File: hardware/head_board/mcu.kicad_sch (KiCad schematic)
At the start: 49 parts, among them SW1 BOOTSEL, U3 RP2040, U4 TVS, U5 W25Q128JVS, U9 74HC2G34, Y1 12MHz

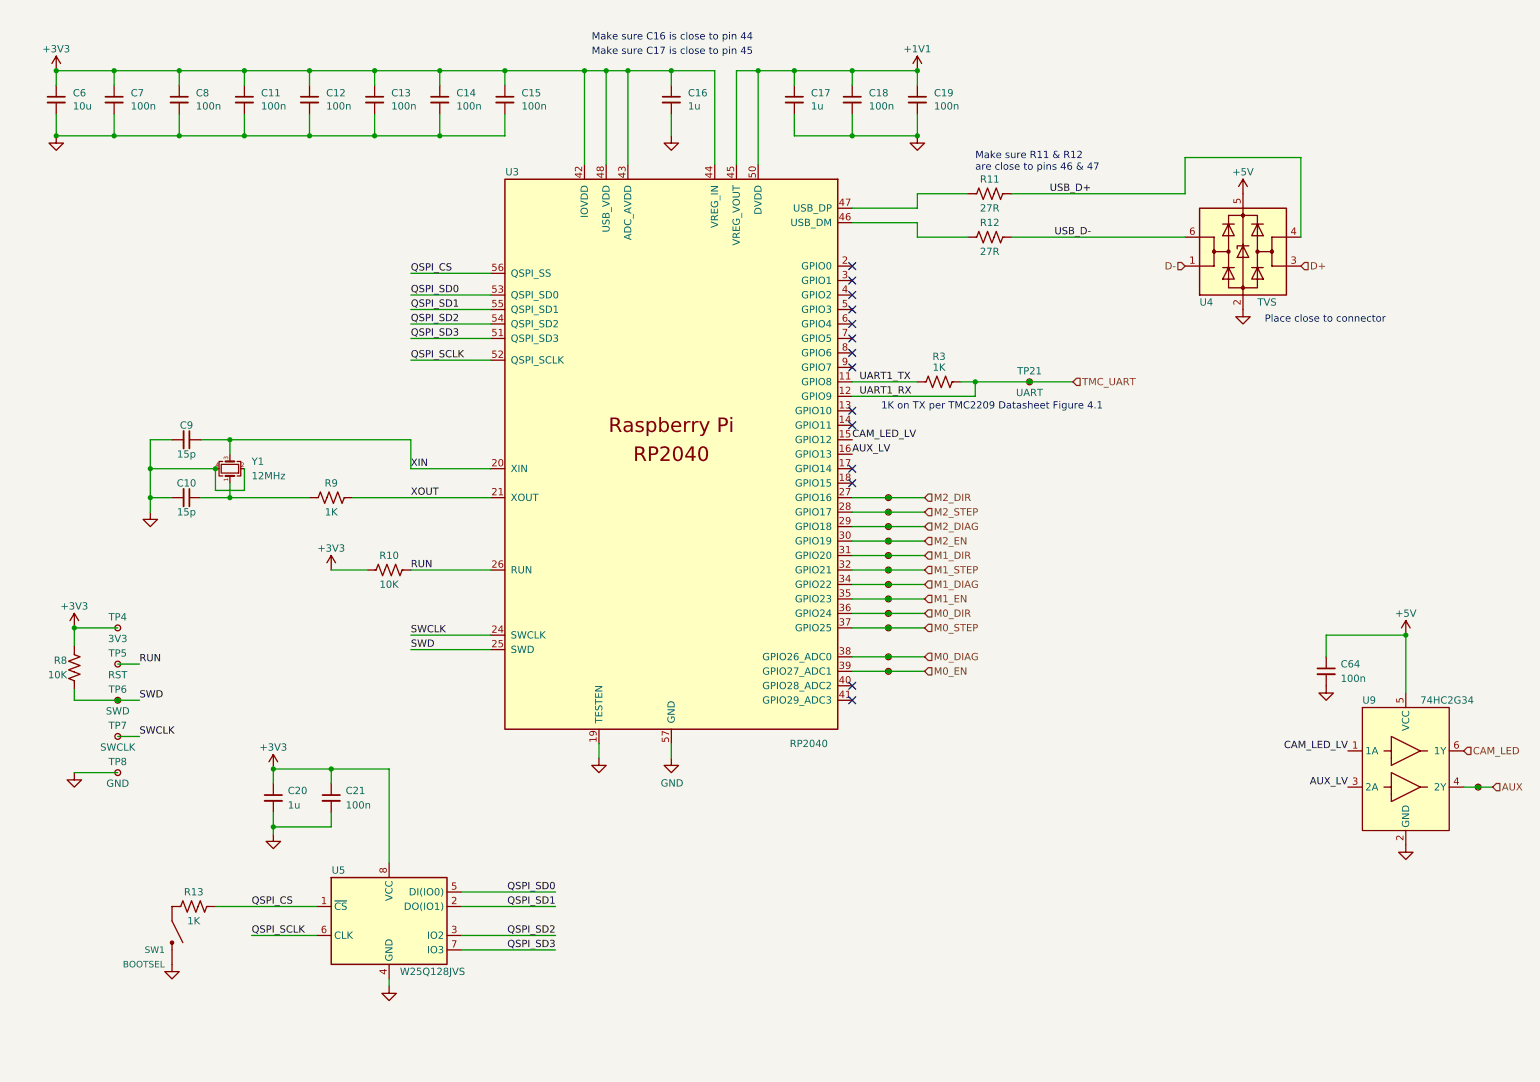
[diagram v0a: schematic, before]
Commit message: v1 revision to the schematic
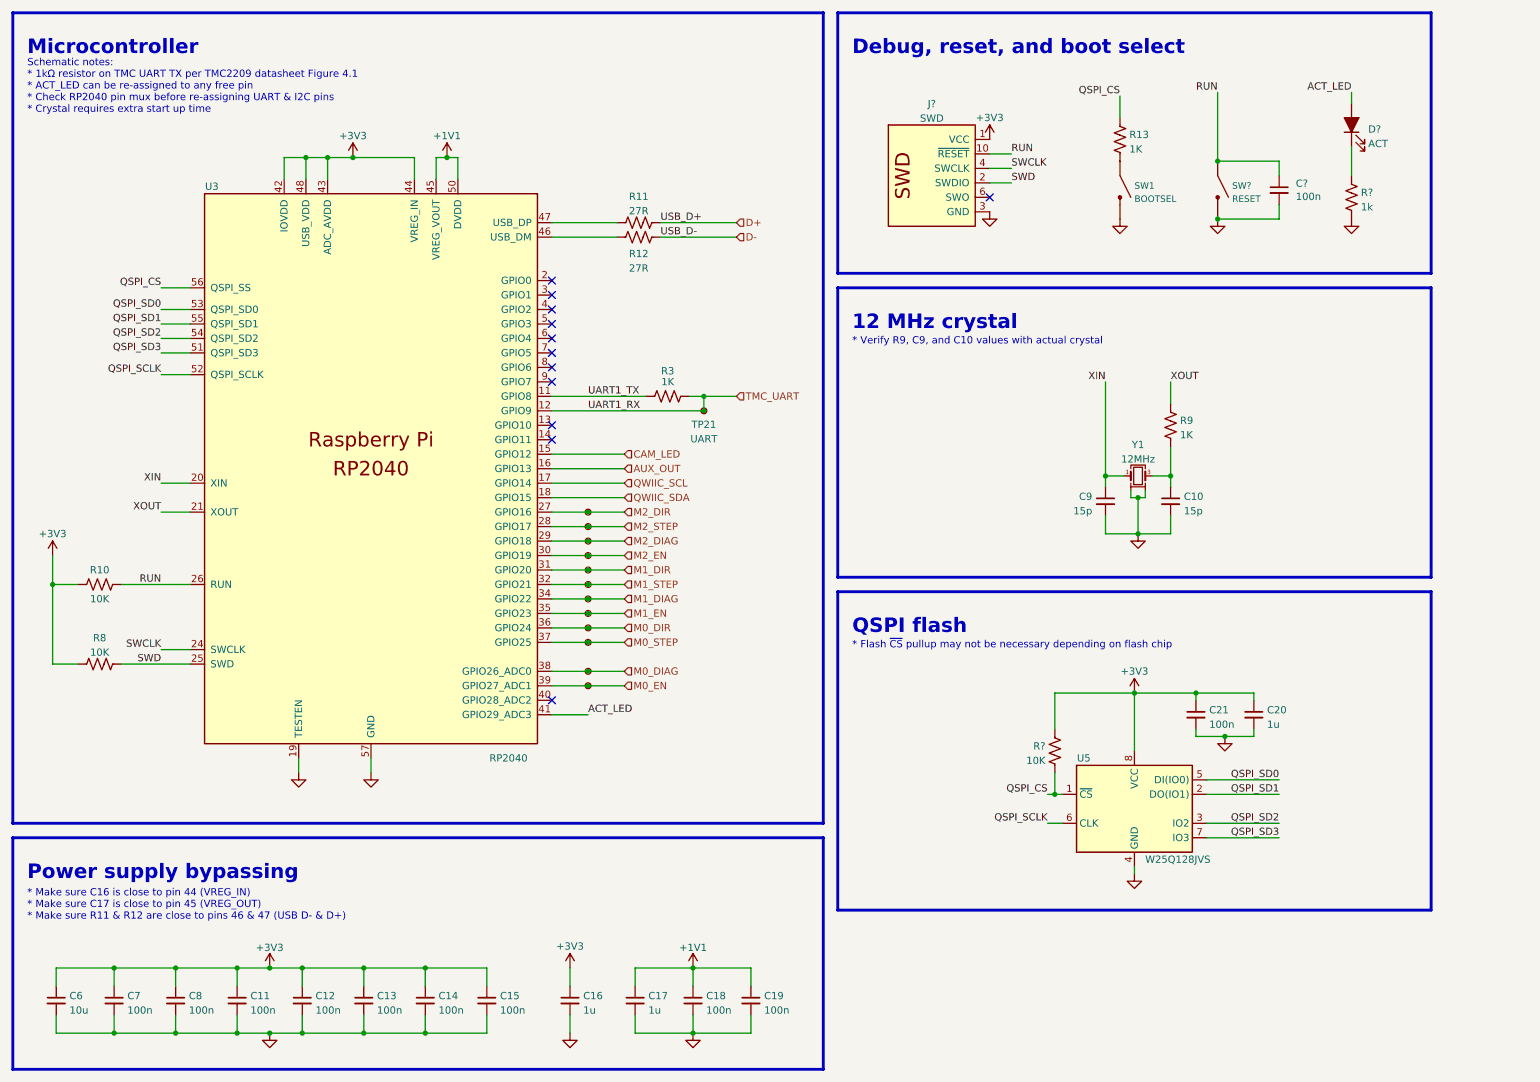
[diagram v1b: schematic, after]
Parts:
- removed C64: 100n, Capacitor_SMD:C_0402_1005Metric_Pad0.74x0.62mm_HandSolder, symbol Device:C_Small
- removed TP22: AUX, TestPoint:TestPoint_Pad_D1.0mm, symbol Connector:TestPoint_Small
- removed TP4: 3V3, TestPoint:TestPoint_Pad_D1.0mm, symbol Connector:TestPoint_Small
- removed TP5: RST, TestPoint:TestPoint_Pad_D1.0mm, symbol Connector:TestPoint_Small
- removed TP6: SWD, TestPoint:TestPoint_Pad_D1.0mm, symbol Connector:TestPoint_Small
- removed TP7: SWCLK, TestPoint:TestPoint_Pad_D1.0mm, symbol Connector:TestPoint_Small
- removed TP8: GND, TestPoint:TestPoint_Pad_D1.0mm, symbol Connector:TestPoint_Small
- removed U4: TVS, Package_TO_SOT_SMD:SOT-23-6, symbol Power_Protection:USBLC6-2SC6
- removed U9: 74HC2G34, Package_TO_SOT_SMD:SOT-363_SC-70-6, symbol winterbloom:74HC2G34
- added C?: 100n, Capacitor_SMD:C_0402_1005Metric_Pad0.74x0.62mm_HandSolder, symbol Device:C_Small
- added D?: ACT, winterbloom:LED_0805_Kingbright_APT2012, symbol Device:LED_Filled
- added J?: SWD, winterbloom:Connector_Cortex_Debug_IDC_2x05_P1.27mm_Vertical_Shrouded_SMD, symbol winterbloom:Conn_SWD
- added R?: 10K, Resistor_SMD:R_0402_1005Metric_Pad0.72x0.64mm_HandSolder, symbol Device:R_US
- added R?: 1k, Resistor_SMD:R_0603_1608Metric_Pad0.98x0.95mm_HandSolder, symbol Device:R_US
- added SW?: RESET, winterbloom:Tactile_Switch_4.2mm, symbol winterbloom:Tactile_Switch
- Y1: symbol Device:Crystal_GND24_Small -> winterbloom:Crystal_12MHz_4Pin
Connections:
- net CAM_LED_LV is gone; now on net CAM_LED: U3.15 (GPIO12)
- net USB_D+ is gone; now on net D+: R11.1
- net USB_D- is gone; now on net D-: R12.1
- net +3V3: now also J?.1 (VCC), R?.2
- net GND: now also C?.2, J?.3 (GND), J?.5 (GND), J?.9 (GNDDetect), R?.2, SW?.2
- net QSPI_CS: now also R?.1
- net RUN: now also C?.1, J?.10 (~{RESET}), SW?.1
- net SWCLK: now also J?.4 (SWCLK)
- net SWD: now also J?.2 (SWDIO)
- net XIN: now also Y1.1; no longer Y1.3
- net at C10.1, R9.2: now also Y1.3; no longer Y1.1
- net QWIIC_SCL: now reaches U3.17 (GPIO14)
- net QWIIC_SDA: now reaches U3.18 (GPIO15)
- net ACT_LED: now reaches U3.41 (GPIO29_ADC3)
- net ACT_LED: now also D?.2 (A)
- net AUX_LV renamed AUX_OUT
- new net: D?.1 (K), R?.1
- no-connect marks 14 -> 12
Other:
- note added: "* Flash ~{CS} pullup may not be necessary depending on flash chip"
- note added: "* Make sure C16 is close to pin 44 (VREG_IN) * Make sure C17 is close to pin 45 (VREG_OUT) * Make sure R11 & R12 are close to pins 46 & 47 (USB D- & D+)"
- note added: "* Verify R9, C9, and C10 values with actual crystal"
- note added: "12 MHz crystal"
- note added: "Debug, reset, and boot select"
- note added: "Microcontroller"
- note added: "Power supply bypassing"
- note added: "QSPI flash"
- note added: "Schematic notes: * 1kΩ resistor on TMC UART TX per TMC2209 datasheet Figure 4.1 * ACT_LED can be re-assigned to any free pin * Check RP2040 pin mux before re-assigning UART & I2C pins * Crystal requires extra start up time"
- note removed: "1K on TX per TMC2209 Datasheet Figure 4.1"
- note removed: "Make sure C16 is close to pin 44"
- note removed: "Make sure C17 is close to pin 45"
- note removed: "Make sure R11 & R12 are close to pins 46 & 47"
- note removed: "Place close to connector"
- company: (none) -> Winterbloom
- title: (none) -> Candela Head
- moved on the sheet: C10, C11, C12, C13, C14, C15, C16, C17, C18, C19, C20, C21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
